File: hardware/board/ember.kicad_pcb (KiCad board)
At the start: 4 copper layers, 150 x 50 mm, 134 parts, among them Q2 2SC1815_C727146, Q3 IRF1018ESTRLPBF, SW1 EC11E18244A5, SW2 SW_Push, SW3 SW_Push, U1 TPS25730D, U10 NT3H2111W0FHKH, U11 DB128L-5.08-2P-BK-S, U12 MAX31865xTP, U13 MAX6675ISA+T, U14 DB128L-5.08-3P-BK-S, U15 TPS56339DDC, U3 TPD6S300A, U4 DB128L-5.08-2P-BK-S, U5 INA226, U6 TMP119AIYBGR, U7 TLP183(GRH-TPL,E(T, U8 W25Q256JVEIQTR, U9 STM32WB55REVx, X1 XL7EL89CKI-111YLC-32M, X2 X201232768KJD2SI

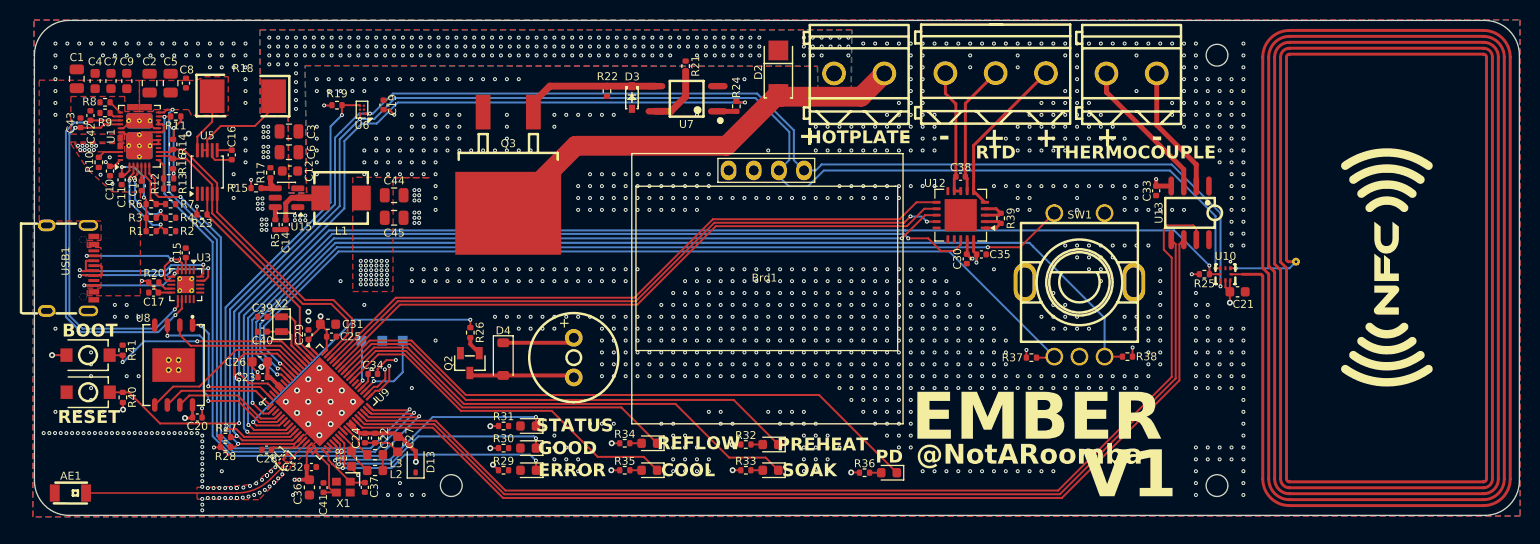
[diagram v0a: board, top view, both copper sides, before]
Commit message: udpate pcb with fixes
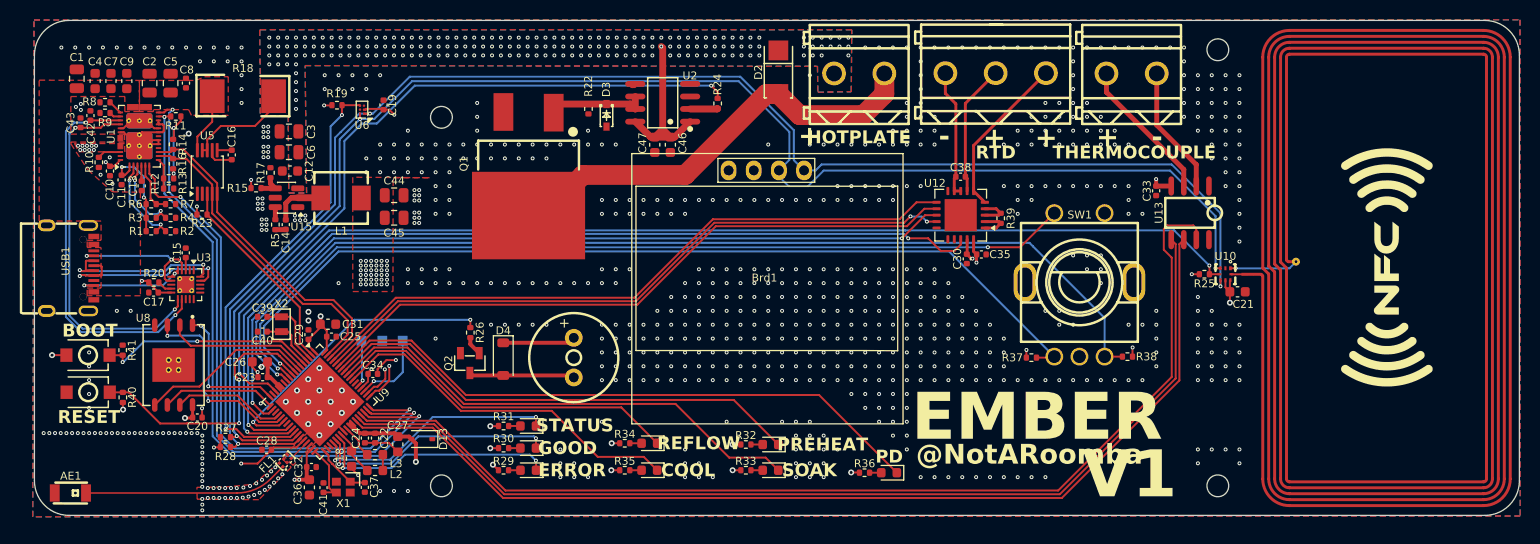
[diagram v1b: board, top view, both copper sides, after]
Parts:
- removed Q3: IRF1018ESTRLPBF, lcsc:TO-263-3_L10.2-W10.7-P5.08-LS16.2-BR
- removed R21: 1K, Resistor_SMD:R_0402_1005Metric
- removed U7: TLP183(GRH-TPL,E(T, lcsc:SOIC-4_L3.6-W4.4-P2.54-LS7.0-TL
- added C46: 4.7uF, Capacitor_SMD:C_0603_1608Metric, F.Cu at (151.7, 76.7)
- added C47: 100nF, Capacitor_SMD:C_0603_1608Metric, F.Cu at (150.1, 76.7)
- added H4: MountingHole, MountingHole:MountingHole_2.2mm_M2, F.Cu at (128.5, 73.9)
- added Q1: IRFS7440TRLPBF, lcsc:TO-263-2_L10.0-W9.1-P5.08-LS15.2-BR, F.Cu at (137.3, 78.6)
- added U2: TC4431EOA, lcsc:SOIC-8_L4.9-W3.9-P1.27-LS6.0-BL, F.Cu at (150.9, 72.4)
- moved D3 3.14 mm to (145.2, 73.7)
- moved R22 2.59 mm to (143.4, 73.0)
- moved D13 2.41 mm to (126.5, 106.4), turned to 180 degrees
- moved R24 1.92 mm to (156.4, 72.5)
- moved H3 0.99 mm to (128.5, 111.1)
- moved H2 0.56 mm to (206.9, 67.0)
- moved H1 0.09 mm to (206.9, 111.1)
- renumbered SWDIO to TP1, SWCLK to TP2, GND to TP3
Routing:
- net PPHV: track 10.8 -> 28.2 mm, vias 191 -> 192
- net Net-(U7-COL): track 6.23 -> 0.00 mm
- net +3.3V: track 71.4 -> 76.4 mm, vias 66 -> 67
- net Net-(D3-K): track 14.0 -> 10.7 mm
- net /HEATBED: track 75.3 -> 73.3 mm
- net /I2C_SCL: track 148.8 -> 150.2 mm
- net /I2C_SDA: track 150.3 -> 151.8 mm
- net Net-(D5-A): track 0.00 -> 1.20 mm
- net Net-(D7-A): track 0.00 -> 1.19 mm
- net Net-(D6-A): track 0.00 -> 1.19 mm
- net Net-(U2-IN): track 1.88 -> 2.80 mm
- net Net-(D2-A): track 45.2 -> 44.6 mm
- net GND: track 24.4 -> 24.6 mm, vias 1180 -> 784
- removed copper zone on In1.Cu, net PPHV
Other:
- board text added: "GND"
- board text added: "SWCLK"
- board text added: "SWDIO"
